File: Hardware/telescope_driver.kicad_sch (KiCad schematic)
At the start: 63 parts, among them J1 GPIO, J2 Battery 12-14V, J3 Stepper_Motor_bipolar, J4 Stepper_Motor_bipolar, U1 TMC2209-LA, U2 TMC2209-LA, U3 LM2678S-12

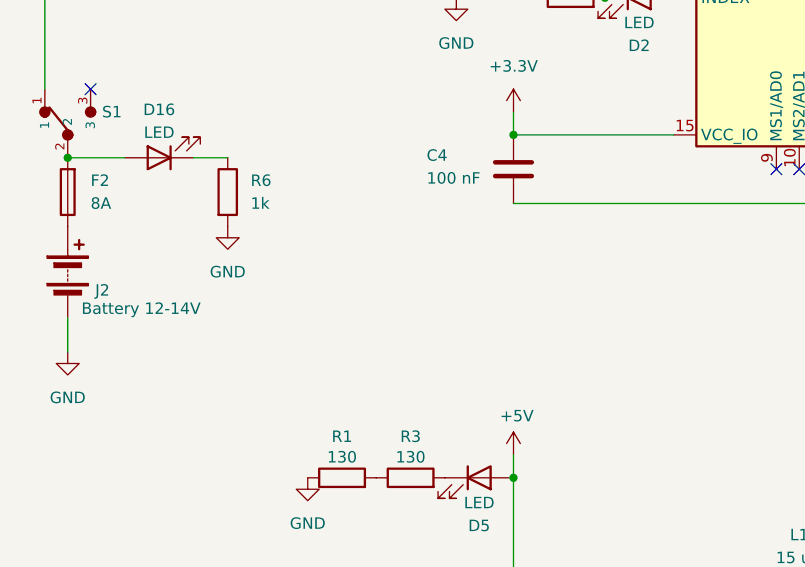
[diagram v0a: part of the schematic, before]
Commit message: parl
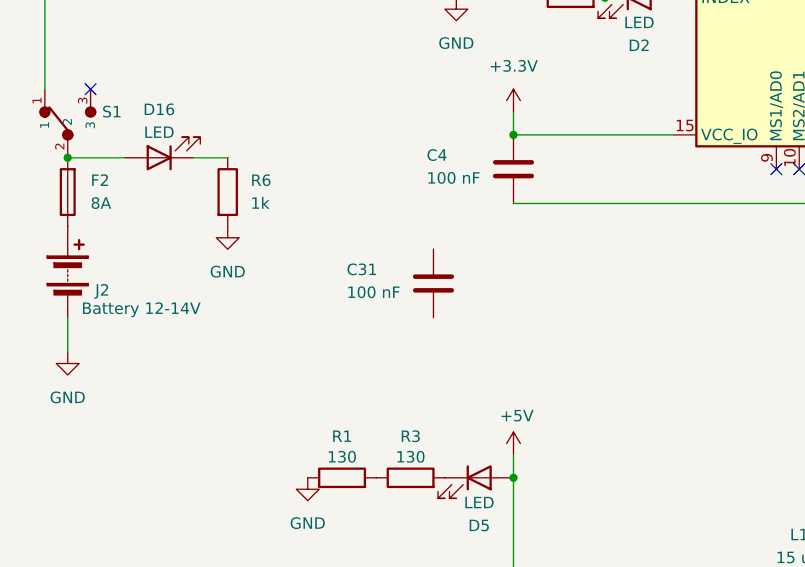
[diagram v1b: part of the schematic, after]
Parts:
- added C31: 100 nF, Capacitor_SMD:C_1206_3216Metric_Pad1.33x1.80mm_HandSolder, symbol Device:C
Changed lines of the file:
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@@
+	)
+	(symbol
+		(lib_id "Device:C")
+		(at 62.23 193.04 180)
+		(unit 1)
+		(exclude_from_sim no)
+		(in_bom yes)
+		(on_board yes)
+		(dnp no)
+		(property "Reference" "C31"
+			(at 52.578 191.516 0)
+			(effects
+				(font
+					(size 1.27 1.27)
+				)
+				(justify right)
+			)
+		)
+		(property "Value" "100 nF"
+			(at 52.578 194.056 0)
+			(effects
+				(font
+					(size 1.27 1.27)
+				)
+				(justify right)
+			)
+		)
+		(property "Footprint" "Capacitor_SMD:C_1206_3216Metric_Pad1.33x1.80mm_HandSolder"
+			(at 61.2648 189.23 0)
+			(effects
+				(font
+					(size 1.27 1.27)
+				)
+				(hide yes)
+			)
+		)
+		(property "Datasheet" "~"
+			(at 62.23 193.04 0)
+			(effects
+				(font
+					(size 1.27 1.27)
+				)
+				(hide yes)
+			)
+		)
+		(property "Description" "Unpolarized capacitor"
+			(at 62.23 193.04 0)
+			(effects
+				(font
+					(size 1.27 1.27)
+				)
+				(hide yes)
+			)
+		)
+		(pin "2"
+		)
+		(pin "1"
+		)
+		(instances
+			(project "telescope_driver"
+				(path "/e63e39d7-6ac0-4ffd-8aa3-1841a4541b55"
+					(reference "C31")
+					(unit 1)
+				)
+			)
+		)
 	)
 	(symbol

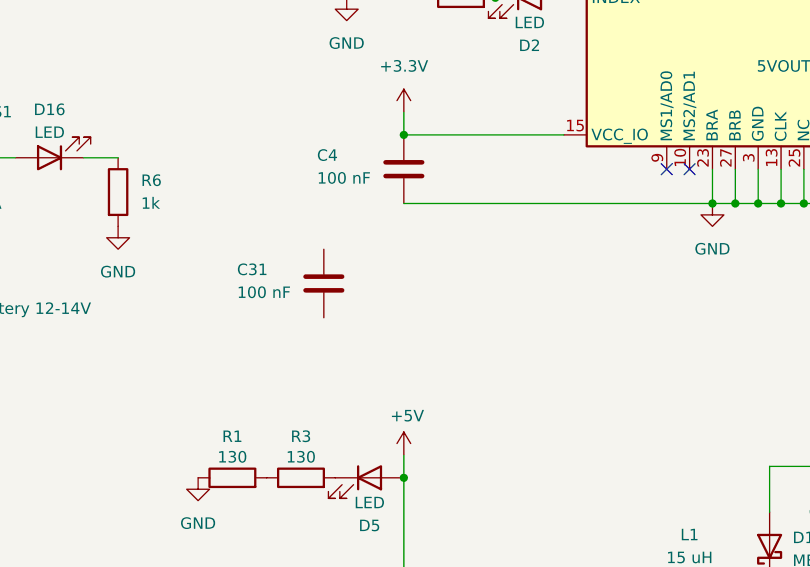
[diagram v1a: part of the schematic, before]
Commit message: ps
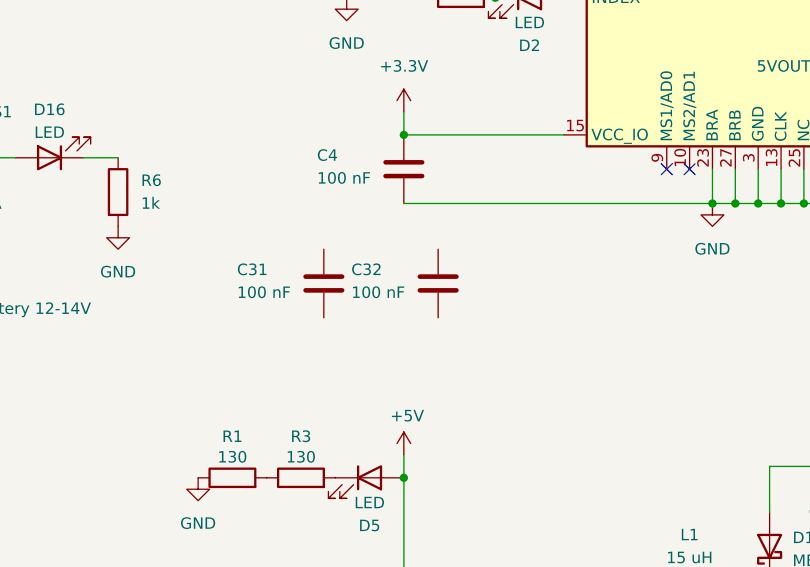
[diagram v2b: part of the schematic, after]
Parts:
- added C32: 100 nF, Capacitor_SMD:C_1206_3216Metric_Pad1.33x1.80mm_HandSolder, symbol Device:C
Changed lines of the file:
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@@
+	)
+	(symbol
+		(lib_id "Device:C")
+		(at 74.93 193.04 180)
+		(unit 1)
+		(exclude_from_sim no)
+		(in_bom yes)
+		(on_board yes)
+		(dnp no)
+		(property "Reference" "C32"
+			(at 65.278 191.516 0)
+			(effects
+				(font
+					(size 1.27 1.27)
+				)
+				(justify right)
+			)
+		)
+		(property "Value" "100 nF"
+			(at 65.278 194.056 0)
+			(effects
+				(font
+					(size 1.27 1.27)
+				)
+				(justify right)
+			)
+		)
+		(property "Footprint" "Capacitor_SMD:C_1206_3216Metric_Pad1.33x1.80mm_HandSolder"
+			(at 73.9648 189.23 0)
+			(effects
+				(font
+					(size 1.27 1.27)
+				)
+				(hide yes)
+			)
+		)
+		(property "Datasheet" "~"
+			(at 74.93 193.04 0)
+			(effects
+				(font
+					(size 1.27 1.27)
+				)
+				(hide yes)
+			)
+		)
+		(property "Description" "Unpolarized capacitor"
+			(at 74.93 193.04 0)
+			(effects
+				(font
+					(size 1.27 1.27)
+				)
+				(hide yes)
+			)
+		)
+		(pin "2"
+		)
+		(pin "1"
+		)
+		(instances
+			(project "telescope_driver"
+				(path "/e63e39d7-6ac0-4ffd-8aa3-1841a4541b55"
+					(reference "C32")
+					(unit 1)
+				)
+			)
+		)
 	)
 	(symbol

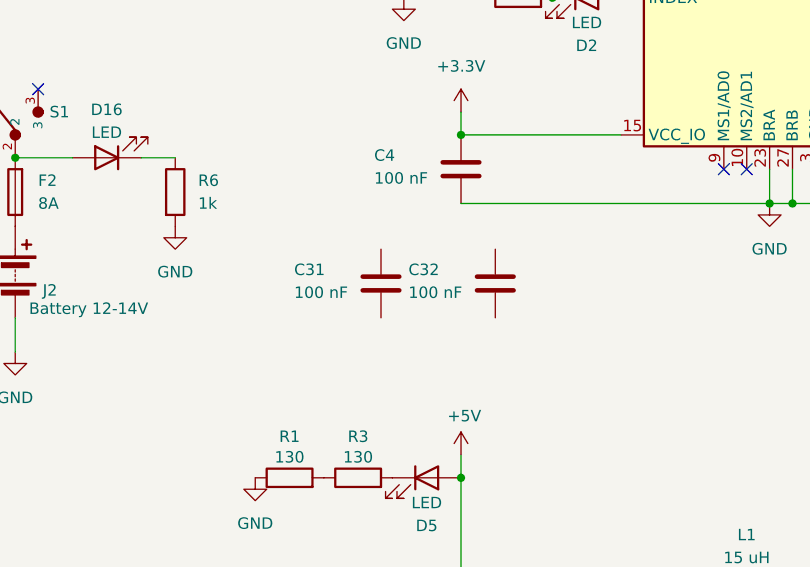
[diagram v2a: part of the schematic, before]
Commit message: finally
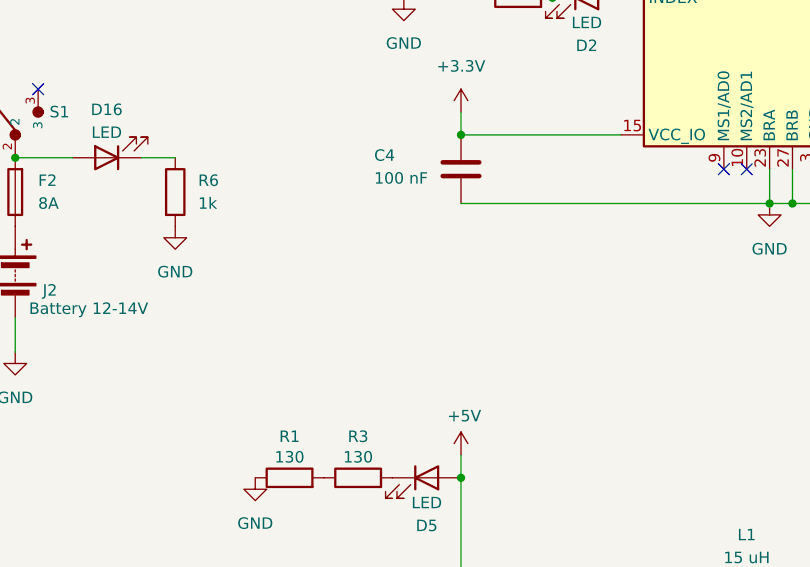
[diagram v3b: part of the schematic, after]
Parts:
- removed C31, C32: 100 nF, Capacitor_SMD:C_1206_3216Metric_Pad1.33x1.80mm_HandSolder, symbol Device:C
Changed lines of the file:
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@@
-	)
-	(symbol
-		(lib_id "Device:C")
-		(at 62.23 193.04 180)
-		(unit 1)
-		(exclude_from_sim no)
-		(in_bom yes)
-		(on_board yes)
-		(dnp no)
-		(property "Reference" "C31"
-			(at 52.578 191.516 0)
-			(effects
-				(font
-					(size 1.27 1.27)
-				)
-				(justify right)
-			)
-		)
-		(property "Value" "100 nF"
-			(at 52.578 194.056 0)
-			(effects
-				(font
-					(size 1.27 1.27)
-				)
-				(justify right)
-			)
-		)
-		(property "Footprint" "Capacitor_SMD:C_1206_3216Metric_Pad1.33x1.80mm_HandSolder"
-			(at 61.2648 189.23 0)
-			(effects
-				(font
-					(size 1.27 1.27)
-				)
-				(hide yes)
-			)
-		)
-		(property "Datasheet" "~"
-			(at 62.23 193.04 0)
-			(effects
-				(font
-					(size 1.27 1.27)
-				)
-				(hide yes)
-			)
-		)
-		(property "Description" "Unpolarized capacitor"
-			(at 62.23 193.04 0)
-			(effects
-				(font
-					(size 1.27 1.27)
-				)
-				(hide yes)
-			)
-		)
-		(pin "2"
-		)
-		(pin "1"
-		)
-		(instances
-			(project "telescope_driver"
-				(path "/e63e39d7-6ac0-4ffd-8aa3-1841a4541b55"
-					(reference "C31")
-					(unit 1)
-				)
-			)
-		)
 	)
 	(symbol
@@
 					(unit 1)
 				)
-			)
-		)
-	)
-	(symbol
-		(lib_id "Device:C")
-		(at 74.93 193.04 180)
-		(unit 1)
-		(exclude_from_sim no)
-		(in_bom yes)
-		(on_board yes)
-		(dnp no)
-		(property "Reference" "C32"
-			(at 65.278 191.516 0)
-			(effects
-				(font
-					(size 1.27 1.27)
-				)
-				(justify right)
-			)
-		)
-		(property "Value" "100 nF"
-			(at 65.278 194.056 0)
-			(effects
-				(font
-					(size 1.27 1.27)
-				)
-				(justify right)
-			)
-		)
-		(property "Footprint" "Capacitor_SMD:C_1206_3216Metric_Pad1.33x1.80mm_HandSolder"
-			(at 73.9648 189.23 0)
-			(effects
-				(font
-					(size 1.27 1.27)
-				)
-				(hide yes)
-			)
-		)
-		(property "Datasheet" "~"
-			(at 74.93 193.04 0)
-			(effects
-				(font
-					(size 1.27 1.27)
-				)
-				(hide yes)
-			)
-		)
-		(property "Description" "Unpolarized capacitor"
-			(at 74.93 193.04 0)
-			(effects
-				(font
-					(size 1.27 1.27)
-				)
-				(hide yes)
-			)
-		)
-		(pin "2"
-		)
-		(pin "1"
-		)
-		(instances
-			(project "telescope_driver"
-				(path "/e63e39d7-6ac0-4ffd-8aa3-1841a4541b55"
-					(reference "C32")
-					(unit 1)
-				)
